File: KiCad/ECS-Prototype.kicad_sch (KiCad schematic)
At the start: 46 parts, among them J1 Connector, J3 FC68131, J4 FC68131, J5 FC68131, K1 RY5W-K, Q1 PN2222A, T1 VB_05-1-12, T2 VB_05-1-12, T3 VB_05-1-12, U2 HLK-5M05, U3 LT1498IN8, U4 MCP602T, U5 MCP602T, U6 MCP602T

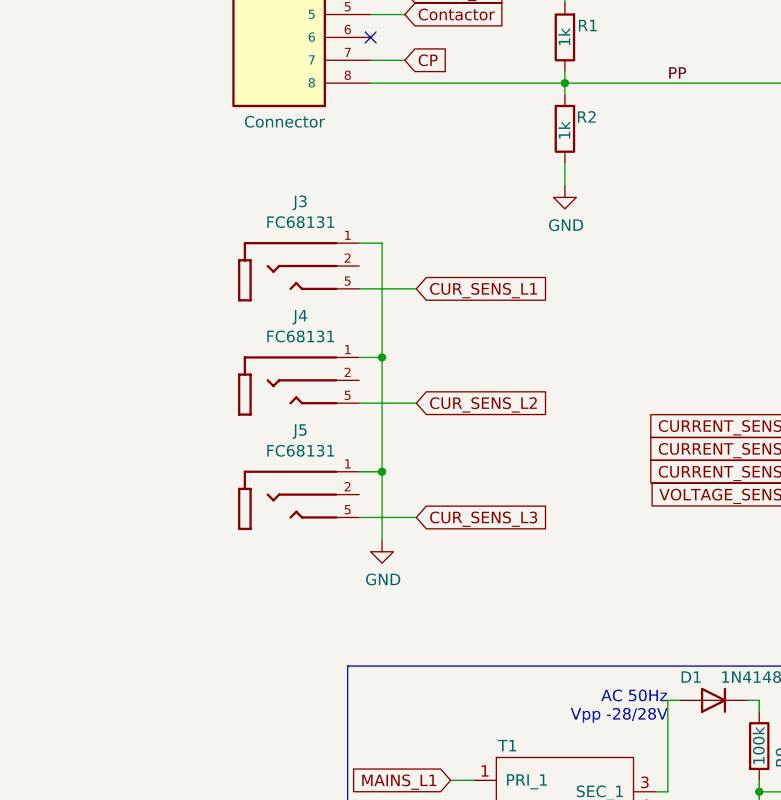
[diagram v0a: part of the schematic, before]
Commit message: modifications for pcb design: version 3
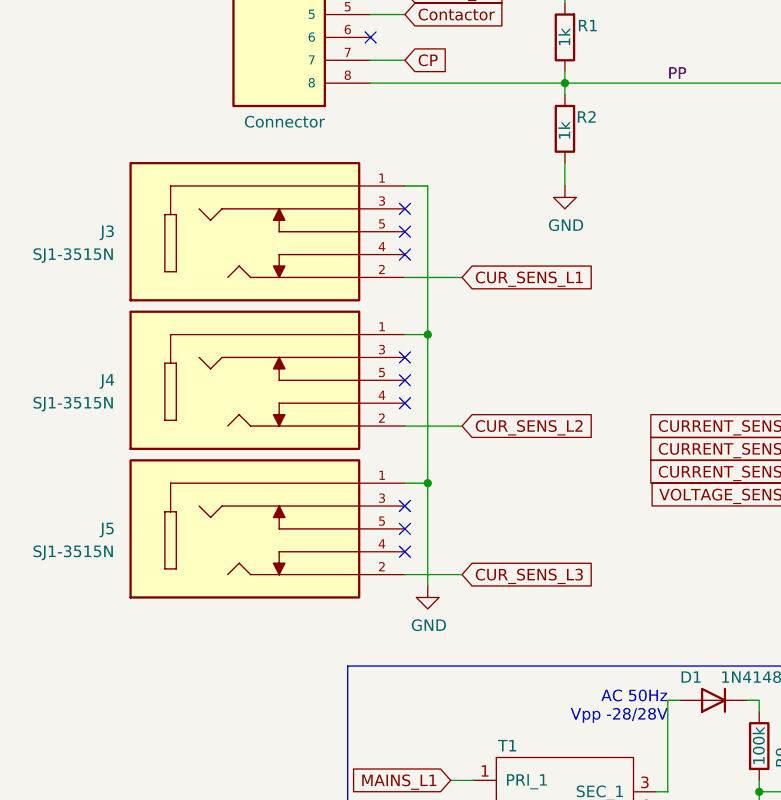
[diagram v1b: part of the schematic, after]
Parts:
- J3, J4, J5: value FC68131 -> SJ1-3515N; footprint DehneEVSEFootPrints:CLIFF_FC68131 -> CUI_SJ1-3515N; symbol ECS-Prototype-rescue:FC68131-DehneEVSESymbols -> SJ1-3515N:SJ1-3515N; MANUFACTURER Cliff -> CUI; PARTREV 5 -> 1.03; STANDARD Manufacturer Recommendations -> Manufacturer recommendation
- T1, T2, T3: footprint DehneEVSEFootPrints:VB_05-1-12 -> ECS-PrototypeFootPrints:VB_05-1-12
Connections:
- net CUR_SENS_L1: now also J3.2; no longer J3.5
- net CUR_SENS_L2: now also J4.2; no longer J4.5
- net CUR_SENS_L3: now also J5.2; no longer J5.5
- no-connect marks 5 -> 14
